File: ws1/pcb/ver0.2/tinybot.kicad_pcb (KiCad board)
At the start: 2 copper layers, 50.3 x 49.8 mm, 18 parts, among them IC1 ATTINY84-P, P1 PWR, P2 PIN Breakout, P3 ICSP, P4 M1, P5 M2, U1 LD1117S33TR, U2 L293D

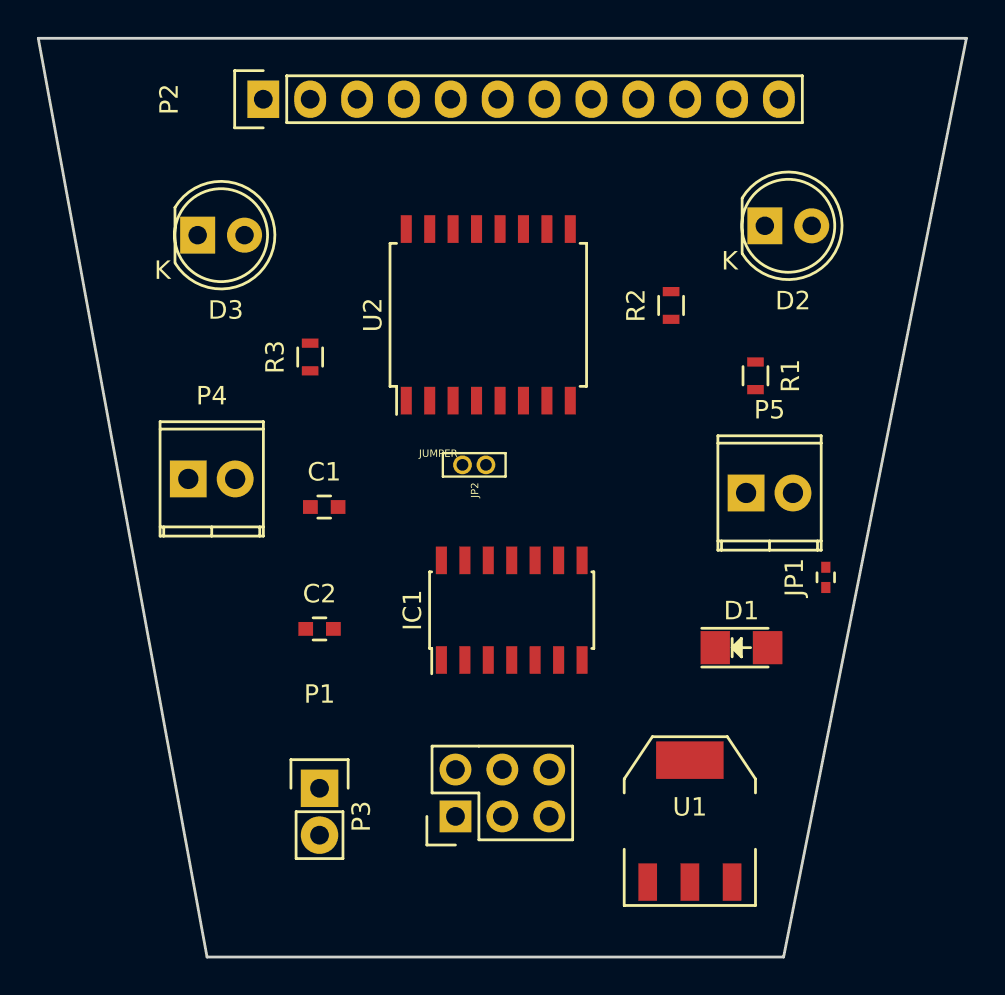
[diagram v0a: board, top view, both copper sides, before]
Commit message: updated
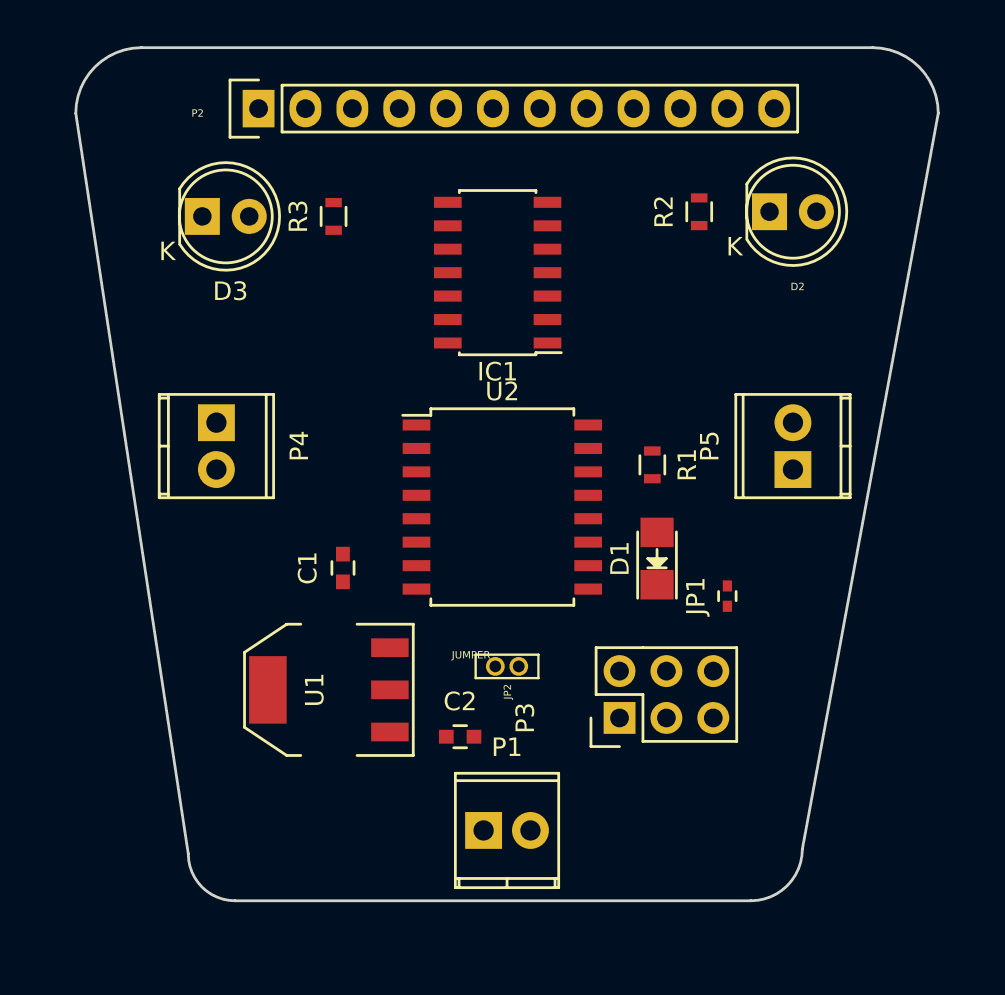
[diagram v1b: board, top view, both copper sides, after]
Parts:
- P1: footprint Pin_Headers:Pin_Header_Straight_1x02 -> Terminal_Blocks:TerminalBlock_Pheonix_MPT-2.54mm_2pol
- moved U1 20.8 mm to (133.6, 98.8), turned to 90 degrees
- moved IC1 18.3 mm to (142.7, 76.2), turned to 180 degrees
- moved JP2 11.1 mm to (143.3, 97.5)
- moved U2 10.4 mm to (143.0, 88.9), turned to 0 degrees
- moved P3 10.4 mm to (149.4, 100.3)
- moved C2 9.60 mm to (140.7, 101.3)
- moved P1 9.18 mm to (142.0, 106.4)
- moved R3 7.73 mm to (133.9, 73.2)
- moved R1 7.38 mm to (151.1, 86.6)
- moved D1 6.65 mm to (151.4, 91.7), turned to 90 degrees
- moved JP1 5.43 mm to (155.2, 93.7)
- moved R2 5.30 mm to (153.7, 72.9)
- moved C1 3.45 mm to (134.4, 92.2), turned to 90 degrees
- moved P4 3.41 mm to (127.5, 84.3), turned to 270 degrees
- moved P5 2.84 mm to (158.8, 86.9), turned to 90 degrees
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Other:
- board size 50.3 x 49.8 mm -> 46.7 x 46.2 mm
